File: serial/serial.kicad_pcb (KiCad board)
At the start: 2 copper layers, 24 x 12 mm, 8 parts, among them J2 Conn_02x03_Odd_Even, Q1 BSS138

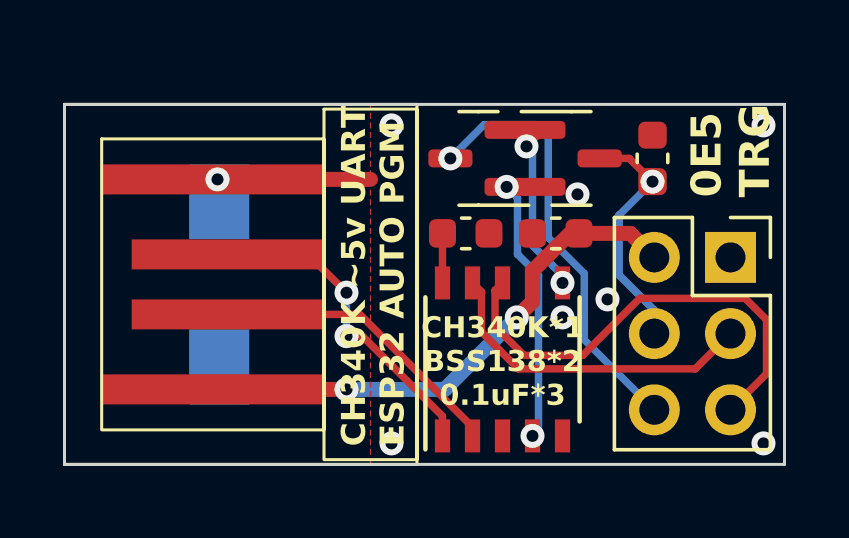
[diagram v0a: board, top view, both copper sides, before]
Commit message: -
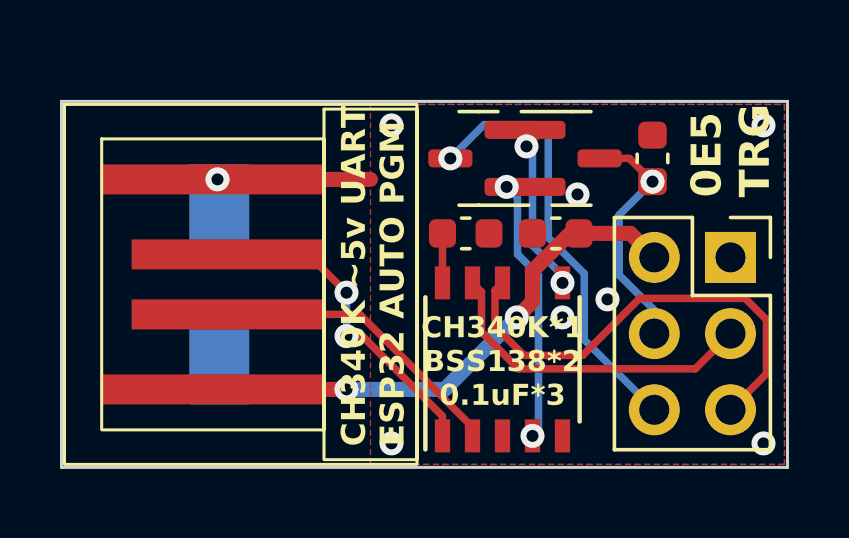
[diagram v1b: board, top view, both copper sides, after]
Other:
- board size 24 x 12 mm -> 24.2 x 12.2 mm

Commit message: -
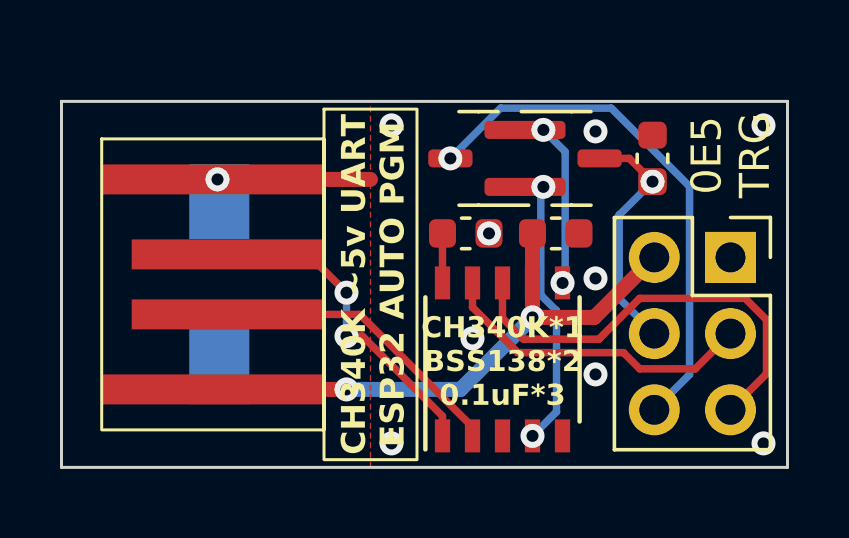
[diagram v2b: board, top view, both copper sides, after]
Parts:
- turned 0u1 to 0 degrees
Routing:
- net Net-(J2-Pin_6): track 14.5 -> 17.7 mm
- net Net-(J2-Pin_2): track 17.8 -> 19.3 mm
- net Net-(J2-Pin_5): track 15.6 -> 14.6 mm
- net Net-(Q1-G): track 5.84 -> 6.66 mm
- net Net-(J2-Pin_1): track 5.26 -> 5.10 mm, vias 8 -> 10
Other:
- board text added: "JLCJLCJLCJLC"
